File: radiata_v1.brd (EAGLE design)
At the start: 80 x 80 mm, 128 parts, among them IC2 MEGA48/88/168-AU, Q1 FA-20H

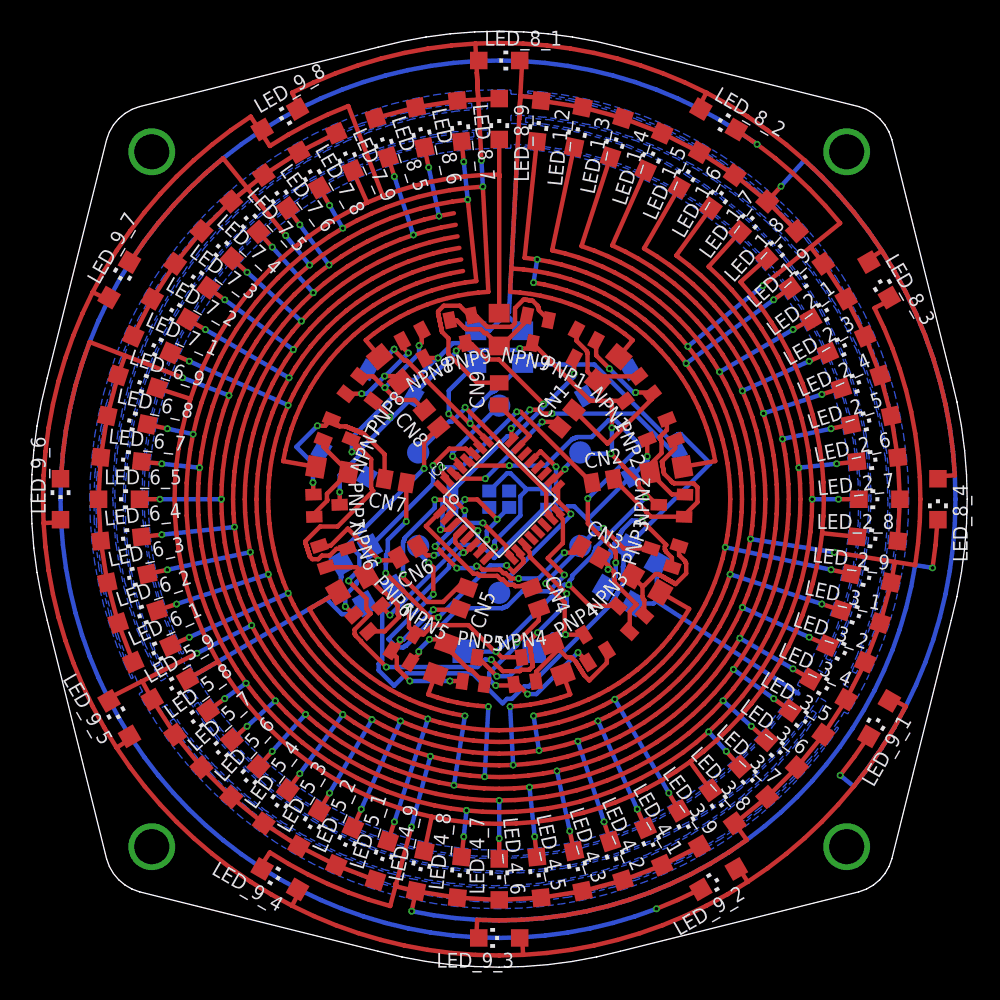
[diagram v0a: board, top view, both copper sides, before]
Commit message: final versions of board and schematic
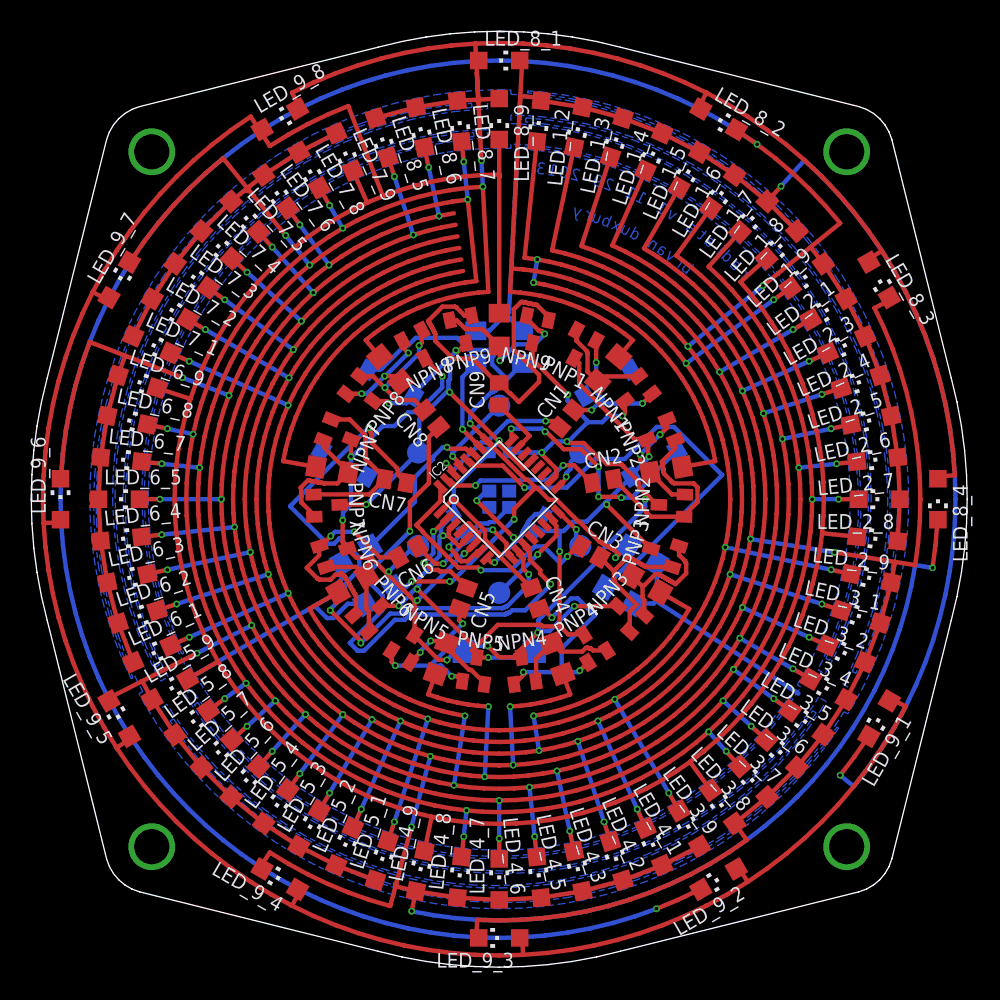
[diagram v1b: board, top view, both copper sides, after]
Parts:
- removed SCL: PTR1TP19R, testpad:TP19R
- added C3: (no value), rcl:C0603
- added SCK: PTR1TP19R, testpad:TP19R
- moved GND 16.0 mm to (33.1, 44.0)
- moved VCC 16.0 mm to (33.1, 36.0)
- moved MOSI 13.9 mm to (40.0, 32.0)
- moved MISO 13.9 mm to (46.9, 36.0)
- moved C1 2.07 mm to (36.5, 38.0), turned to 60 degrees
- moved C2 2.07 mm to (43.5, 38.0), turned to 300 degrees
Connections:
- net GND: now also C3.2
- net N$6: now also SCK.TP; no longer SCL.TP
- net VCC: now also C3.1
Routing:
- net PC2: track 89.8 -> 57.7 mm, vias 2 -> 5
- net N$7: track 35.0 -> 3.76 mm, vias 3 -> 1
- net PD6: track 25.3 -> 52.8 mm
- net N$8: track 18.2 -> 8.58 mm
- net PD4: track 18.0 -> 9.31 mm
- net N$6: track 12.1 -> 3.80 mm
- net PC5: track 32.9 -> 40.7 mm, vias 3 -> 1
- net N$29: track 22.4 -> 29.4 mm
- net PD7: track 53.8 -> 47.0 mm, vias 6 -> 2
- net N$14: track 19.1 -> 13.7 mm, vias 2 -> 0
- net N$28: track 8.84 -> 13.6 mm, vias 0 -> 2
- net PD1: track 18.6 -> 13.9 mm
- net N$10: track 17.4 -> 12.9 mm, vias 2 -> 3
- net N$20: track 14.8 -> 18.3 mm
- net PC1: track 17.5 -> 20.9 mm, vias 3 -> 5
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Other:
- board text added: "-"
- board text added: "0"
- board text added: "1"
- board text added: "2"
- board text added: "3"
- board text added: "9"
- board text added: "a"
- board text added: "b"
- board text added: "d"
- board text added: "i"
- board text added: "n"
- board text added: "r"
- board text added: "t"
- board text added: "u"
- board text added: "v"
- board text added: "x"
- board text added: "y"
